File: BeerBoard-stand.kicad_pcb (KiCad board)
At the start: 2 copper layers, 45 x 30 mm, 12 parts, among them J1 Conn_02x04_Odd_Even

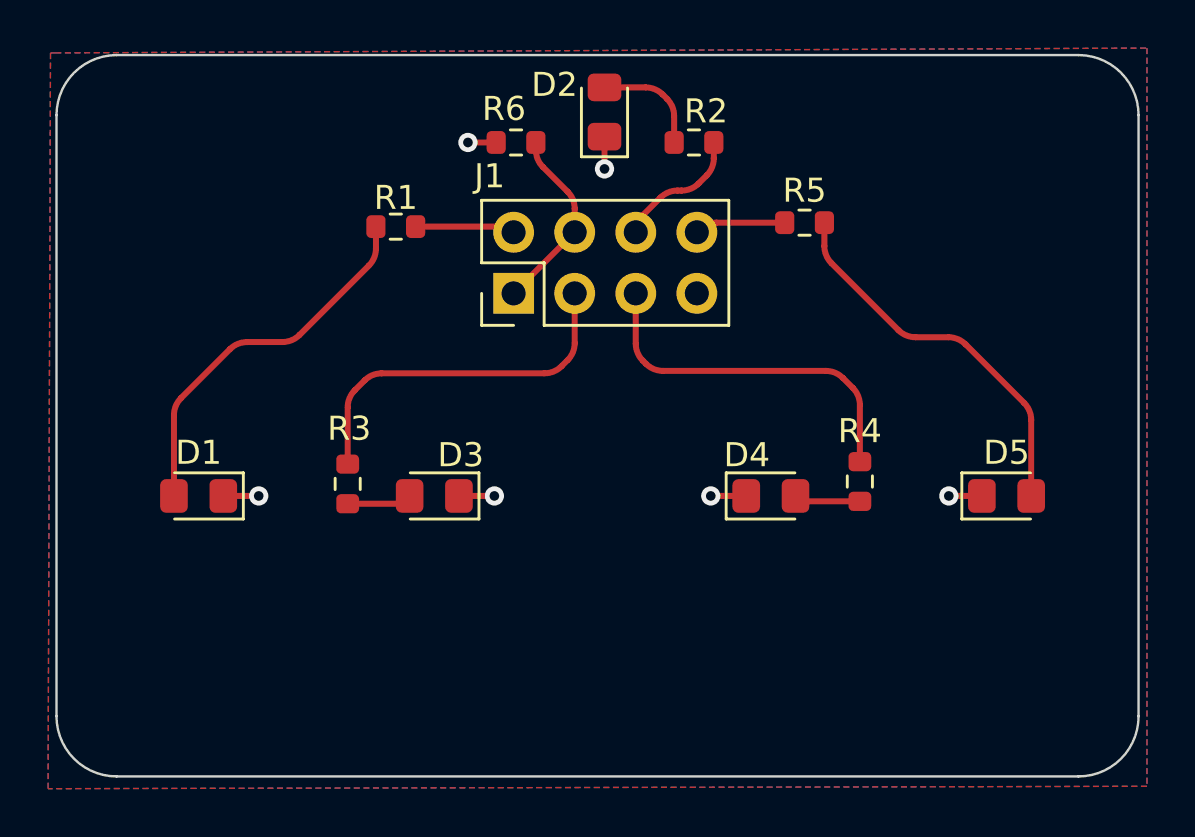
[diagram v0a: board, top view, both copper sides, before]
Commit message: Some updates, added images
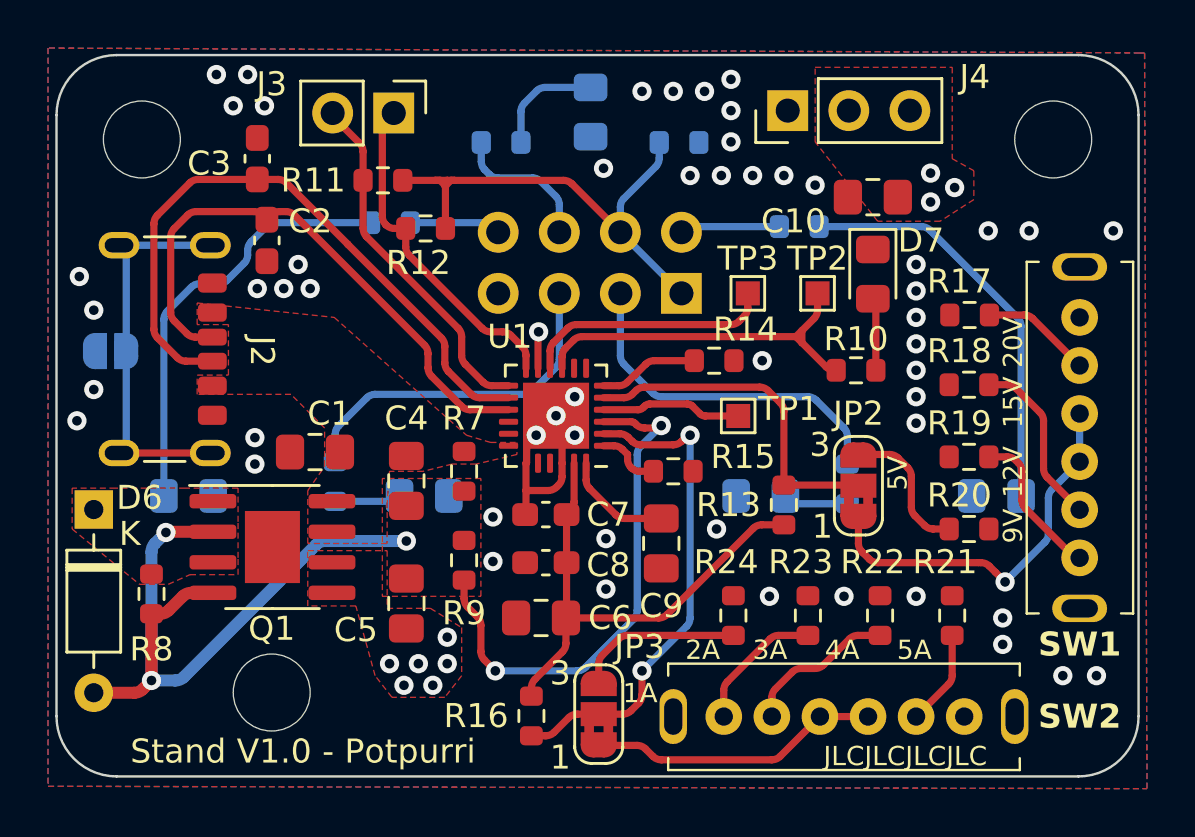
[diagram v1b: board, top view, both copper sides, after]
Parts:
- added C1: 3u3, Capacitor_SMD:C_0805_2012Metric_Pad1.18x1.45mm_HandSolder, F.Cu at (105.6, 61.8)
- added C10: 3u3, Capacitor_SMD:C_0805_2012Metric_Pad1.18x1.45mm_HandSolder, F.Cu at (128.8, 51.2)
- added C2: 390p, Capacitor_SMD:C_0603_1608Metric_Pad1.08x0.95mm_HandSolder, F.Cu at (103.6, 53.0)
- added C3: 390p, Capacitor_SMD:C_0603_1608Metric_Pad1.08x0.95mm_HandSolder, F.Cu at (103.2, 49.6)
- added C4: 1u, Capacitor_SMD:C_0805_2012Metric_Pad1.18x1.45mm_HandSolder, F.Cu at (109.4, 63.0)
- added C5: 1u, Capacitor_SMD:C_0805_2012Metric_Pad1.18x1.45mm_HandSolder, F.Cu at (109.4, 68.1)
- added C6: 1u, Capacitor_SMD:C_0805_2012Metric_Pad1.18x1.45mm_HandSolder, F.Cu at (115.0, 68.7)
- added C7: 100n, Capacitor_SMD:C_0603_1608Metric_Pad1.08x0.95mm_HandSolder, F.Cu at (115.2, 64.4)
- added C8: 100n, Capacitor_SMD:C_0603_1608Metric_Pad1.08x0.95mm_HandSolder, F.Cu at (115.2, 66.4)
- added C9: 1u, Capacitor_SMD:C_0805_2012Metric_Pad1.18x1.45mm_HandSolder, F.Cu at (120.0, 65.6)
- added D6: D_Zener, Diode_THT:D_DO-35_SOD27_P7.62mm_Horizontal, F.Cu at (96.4, 64.2)
- added D7: LED, LED_SMD:LED_0805_2012Metric_Pad1.15x1.40mm_HandSolder, F.Cu at (128.8, 54.4)
- added H1: MountingHole, MountingHole:MountingHole_3.2mm_M3, F.Cu at (98.4, 48.8)
- added H2: MountingHole, MountingHole:MountingHole_3.2mm_M3, F.Cu at (136.3, 48.8)
- added H3: MountingHole, MountingHole:MountingHole_3.2mm_M3, F.Cu at (103.8, 71.8)
- added J2: Type-C_6P, Connector_USB:USB_C_Receptacle_GCT_USB4125-xx-x-0190_6P_TopMnt_Horizontal, F.Cu at (98.2, 57.5)
- added J3: I2C, Connector_PinHeader_2.54mm:PinHeader_1x02_P2.54mm_Vertical, F.Cu at (108.9, 47.7)
- added J4: Conn_01x03, Connector_PinHeader_2.54mm:PinHeader_1x03_P2.54mm_Vertical, F.Cu at (125.3, 47.6)
- added JP1: SolderJumper_2_Open, Jumper:SolderJumper-2_P1.3mm_Open_RoundedPad1.0x1.5mm, B.Cu at (97.1, 57.6)
- added JP2: SolderJumper_3_Bridged12, Jumper:SolderJumper-3_P1.3mm_Bridged2Bar12_RoundedPad1.0x1.5mm_NumberLabels, F.Cu at (128.2, 63.2)
- added JP3: SolderJumper_3_Bridged12, Jumper:SolderJumper-3_P1.3mm_Bridged2Bar12_RoundedPad1.0x1.5mm_NumberLabels, F.Cu at (117.4, 72.7)
- added Q1: DMP3098LSD, Package_SO:SOIC-8-1EP_3.9x4.9mm_P1.27mm_EP2.29x3mm, F.Cu at (103.8, 65.8)
- added R10: 1k, Resistor_SMD:R_0603_1608Metric, F.Cu at (128.1, 58.4)
- added R11: 2k4, Resistor_SMD:R_0603_1608Metric, F.Cu at (108.4, 50.5)
- added R12: 2k4, Resistor_SMD:R_0603_1608Metric, F.Cu at (110.2, 52.5)
- added R13: 5k1, Resistor_SMD:R_0603_1608Metric, F.Cu at (125.1, 64.0)
- added R14: 5k1, Resistor_SMD:R_0603_1608Metric, F.Cu at (122.2, 58.0)
- added R15: 5k1, Resistor_SMD:R_0603_1608Metric, F.Cu at (120.5, 62.6)
- added R16: 5k1, Resistor_SMD:R_0603_1608Metric, F.Cu at (114.6, 72.8)
- added R17: 5k1, Resistor_SMD:R_0603_1608Metric, F.Cu at (132.8, 56.1)
- added R18: 2k4, Resistor_SMD:R_0603_1608Metric, F.Cu at (132.8, 59.0)
- added R19: 1k, Resistor_SMD:R_0603_1608Metric, F.Cu at (132.8, 62.0)
- added R20: 0, Resistor_SMD:R_0603_1608Metric, F.Cu at (132.8, 65.0)
- added R21: 10k, Resistor_SMD:R_0603_1608Metric, F.Cu at (132.1, 68.6)
- added R22: 5k1, Resistor_SMD:R_0603_1608Metric, F.Cu at (129.1, 68.6)
- added R23: 2k4, Resistor_SMD:R_0603_1608Metric, F.Cu at (126.1, 68.6)
- added R24: 1k, Resistor_SMD:R_0603_1608Metric, F.Cu at (123.0, 68.6)
- added R7: 10k, Resistor_SMD:R_0603_1608Metric, F.Cu at (111.8, 62.6)
- added R8: 50K, Resistor_SMD:R_0603_1608Metric, F.Cu at (98.8, 67.7)
- added R9: 1K, Resistor_SMD:R_0603_1608Metric, F.Cu at (111.8, 66.3)
- added SW1: ~, USB:SK-14D01-G 6, F.Cu at (137.4, 61.2)
- added SW2: ~, USB:SK-14D01-G 6, F.Cu at (127.6, 72.8)
- added TP1: TestPoint, TestPoint:TestPoint_Pad_1.0x1.0mm, F.Cu at (123.2, 60.3)
- added TP2: TestPoint, TestPoint:TestPoint_Pad_1.0x1.0mm, F.Cu at (126.5, 55.2)
- added TP3: TestPoint, TestPoint:TestPoint_Pad_1.0x1.0mm, F.Cu at (123.6, 55.2)
- added U1: CYPD3177-24LQ, Package_DFN_QFN:QFN-24-1EP_4x4mm_P0.5mm_EP2.75x2.75mm, F.Cu at (115.6, 60.3)
- D1, D2, D3, D4, D5, J1, R1, R2, R3, R4, R5: moved to B.Cu
- R6: value 100k -> 50k; moved to B.Cu
- moved D5 34.0 mm to (100.3, 63.6), turned to 180 degrees
- moved D1 33.2 mm to (133.9, 63.6), turned to 0 degrees
- moved R4 21.8 mm to (106.4, 63.0)
- moved R3 20.8 mm to (127.7, 63.1)
- moved R5 17.2 mm to (108.7, 52.3), turned to 0 degrees
- moved R1 16.8 mm to (125.7, 52.4), turned to 180 degrees
- moved D4 14.4 mm to (110.1, 63.6), turned to 180 degrees
- moved D3 13.6 mm to (124.1, 63.6), turned to 0 degrees
- moved R2 8.02 mm to (113.3, 48.9), turned to 180 degrees
- moved J1 6.98 mm to (120.8, 55.2)
- moved R6 6.78 mm to (120.7, 48.9), turned to 0 degrees
- moved D2 0.58 mm to (117.1, 47.7)
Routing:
- net Net-(D6-A): track 0.00 -> 29.6 mm, vias 0 -> 3
- net CC2: track 0.00 -> 27.3 mm
- net CC1: track 0.00 -> 24.1 mm
- net Net-(U1-VBUS_FET_EN): track 0.00 -> 21.7 mm, vias 0 -> 2
- net +3V3: track 0.00 -> 21.1 mm
- net Net-(JP3-C): track 0.00 -> 20.8 mm, vias 0 -> 2
- net Net-(J2-SHIELD): track 0.00 -> 16.5 mm
- net Net-(JP2-A): track 0.00 -> 16.1 mm, vias 0 -> 1
- net Net-(U1-FAULT): track 0.00 -> 15.5 mm
- net Net-(J3-Pin_2): track 0.00 -> 14.8 mm
- net Net-(JP2-C): track 0.00 -> 14.3 mm
- net Net-(J3-Pin_1): track 0.00 -> 14.0 mm
- net PB14: track 7.90 -> 21.0 mm
- net Net-(JP3-A): track 0.00 -> 12.1 mm
- net Net-(U1-FLIP): track 0.00 -> 10.4 mm
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- added copper zone on F.Cu, net +VSW
- added copper zone on In2.Cu, net +VSW
- added copper zone on In1.Cu, net GND
- added copper zone on F.Cu, net Net-(D6-A)
- added copper zone on F.Cu, net Net-(D6-K)
- added copper zone on F.Cu, net VBUS
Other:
- copper layers 2 -> 4
- board text added: "12V"
- board text added: "15V"
- board text added: "1A"
- board text added: "20V"
- board text added: "2A"
- board text added: "3A"
- board text added: "4A"
- board text added: "5A"
- board text added: "5V"
- board text added: "9V"
- board text added: "JLCJLCJLCJLC"
- board text added: "Stand V1.0 - Potpurri"
